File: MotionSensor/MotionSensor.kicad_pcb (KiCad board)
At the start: 2 copper layers, 90 x 26.2 mm, 18 parts, among them J1 SSD1306 Display, SW1 TL3301AF160QG, SW2 TL3301AF160QG, SW3 TL3301AF160QG, U1 XIAO-ESP32-C6, U2 XIAO 24GHZ MMWAVE SENSOR

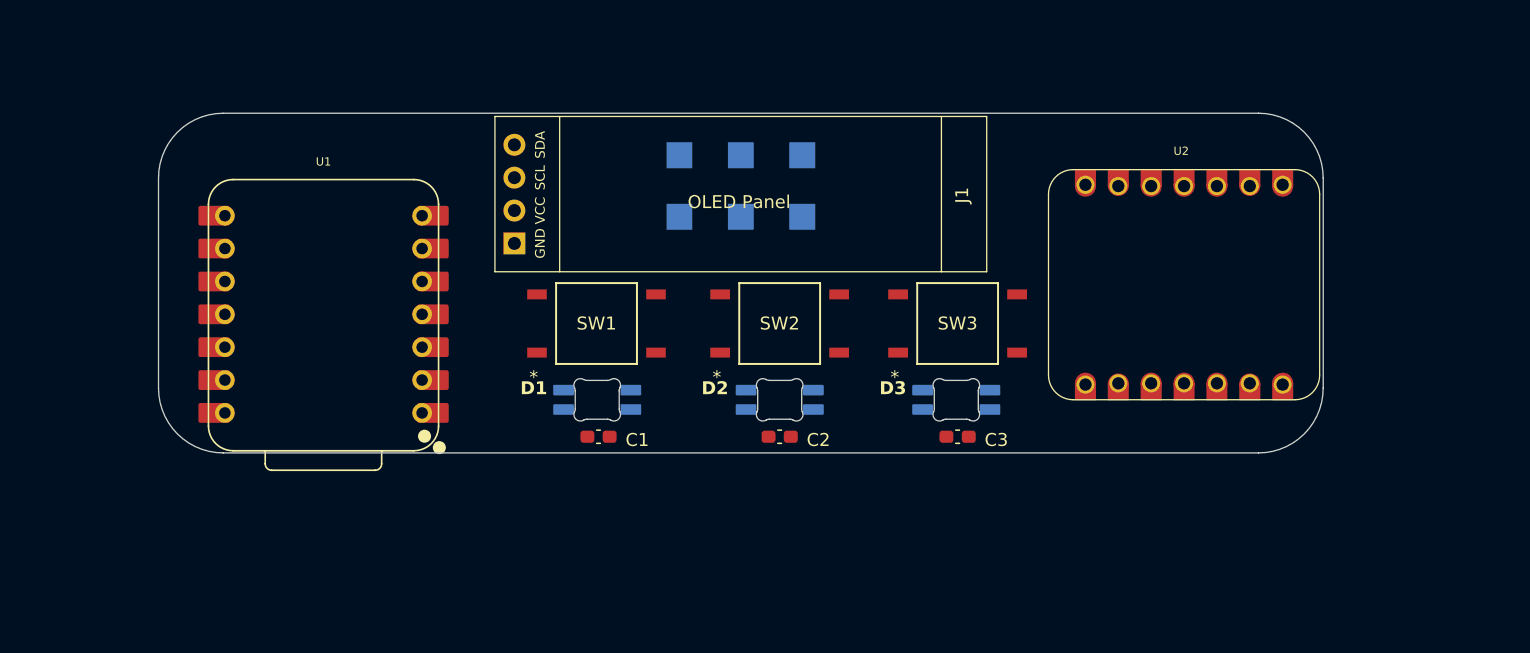
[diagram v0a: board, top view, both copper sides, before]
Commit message: C
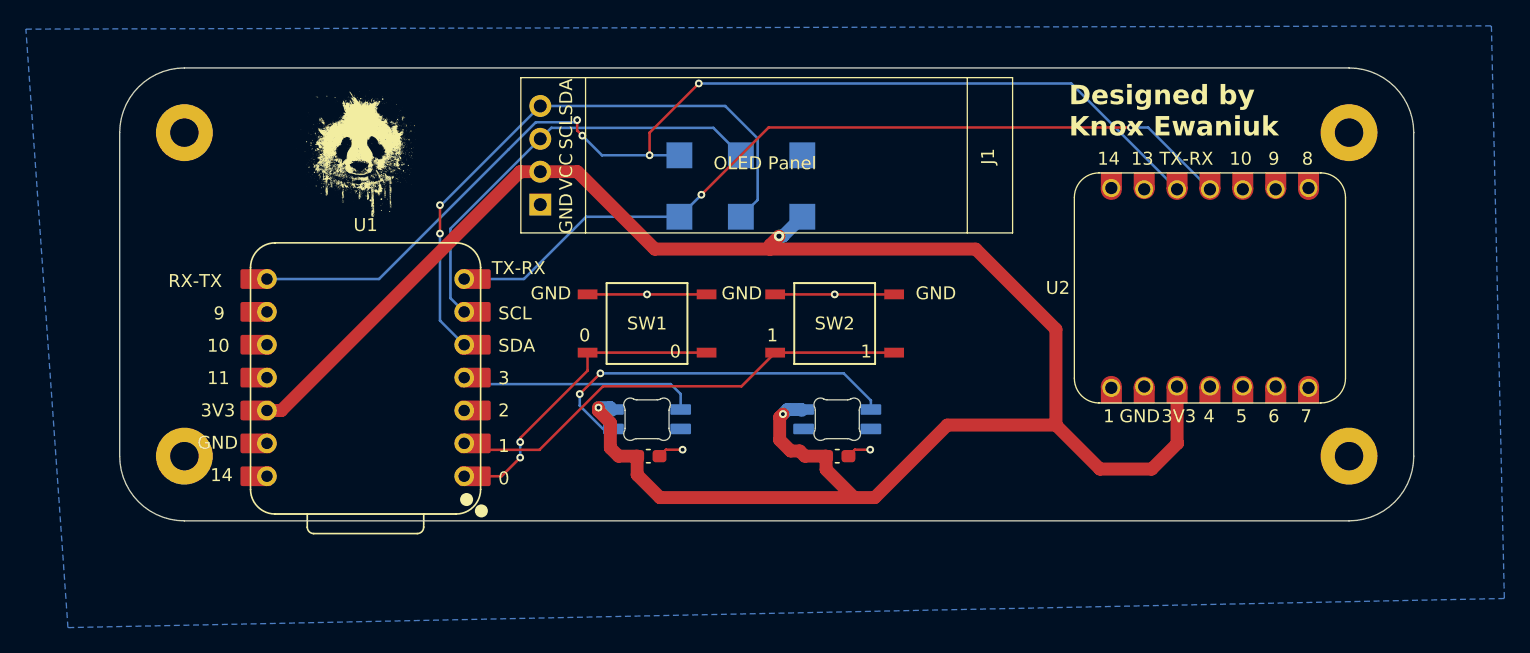
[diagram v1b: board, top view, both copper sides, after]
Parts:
- removed C3: 0.1uF, Capacitor_SMD:C_0603_1608Metric_Pad1.08x0.95mm_HandSolder
- removed D3: SK6812MINI-E, FS:SK6812MINI-E_fixed
- removed SW3: TL3301AF160QG, FS:TL3301_A_G_EWI
- added G***: LOGO, Pictures:Panda_negative3, F.Cu at (98.8, 56.4)
- added G***: LOGO, LOGO, B.Cu at (144.8, 65.6)
- added H1: M2, MountingHole:MountingHole_2.2mm_M2_Pad, F.Cu at (85.2, 55.0)
- added H2: M2, MountingHole:MountingHole_2.2mm_M2_Pad, F.Cu at (85.2, 80.0)
- added H3: M2, MountingHole:MountingHole_2.2mm_M2_Pad, F.Cu at (175.2, 55.0)
- added H4: M2, MountingHole:MountingHole_2.2mm_M2_Pad, F.Cu at (175.2, 80.0)
- moved U1 5.87 mm to (99.2, 73.9)
- moved C2 4.70 mm to (135.7, 80.0)
- moved D2 4.70 mm to (135.7, 77.2)
- moved SW2 4.25 mm to (135.5, 69.8)
- moved C1 4.13 mm to (121.1, 80.0)
- moved D1 4.13 mm to (121.0, 77.2)
- moved SW1 3.90 mm to (121.0, 69.8)
- moved J1 3.61 mm to (149.2, 62.8)
- moved U2 2.02 mm to (164.5, 67.0), turned to 90 degrees
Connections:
- net D0 renamed 0
- net D1 renamed 1
- net D3 renamed 3
- D2 pad 2: Net-(D2-DOUT) -> unconnected-(D2-DOUT-Pad2)
- U1 pad 3: D2 -> unconnected-(U1-GPIO2/A2/D2-Pad3)
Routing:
- net +3V3: track 0.00 -> 155.9 mm, vias 0 -> 3
- net RX-TX: track 0.00 -> 86.0 mm, vias 0 -> 4
- net TX-RX: track 0.00 -> 64.5 mm, vias 0 -> 2
- net SDA: track 0.00 -> 46.9 mm, vias 0 -> 2
- net 1: track 0.00 -> 36.5 mm
- net SCL: track 0.00 -> 33.4 mm
- net Net-(D1-DOUT): track 0.00 -> 29.0 mm, vias 0 -> 2
- net 0: track 0.00 -> 24.4 mm, vias 0 -> 2
- net GND: track 0.00 -> 22.3 mm, vias 0 -> 4
- net 3: track 0.00 -> 18.5 mm
- added copper zone on B.Cu, net GND
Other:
- board size 90 x 26.2 mm -> 100 x 35 mm
- board text added: "0"
- board text added: "1"
- board text added: "10"
- board text added: "11"
- board text added: "13"
- board text added: "14"
- board text added: "2"
- board text added: "3"
- board text added: "3V3"
- board text added: "4"
- board text added: "5"
- board text added: "6"
- board text added: "7"
- board text added: "8"
- board text added: "9"
- board text added: "Designed by Knox Ewaniuk"
- board text added: "GND"
- board text added: "RX-TX"
- board text added: "SCL"
- board text added: "SDA"
- board text added: "TX-RX"
